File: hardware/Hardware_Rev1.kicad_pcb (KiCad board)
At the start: 2 copper layers, 120.7 x 44.5 mm, 56 parts, among them J1 RJ45_LED_Shielded, J2 6P6C, Q1 BUK9M9R5-40HX, Q2 BUK9M9R5-40HX, Q3 BUK9M9R5-40HX, U1 LT1910, U2 LT1910, U3 OKI, U4 LT1910, U5 TSR_1-2450, U6 Teensy4.1_DEV-16771

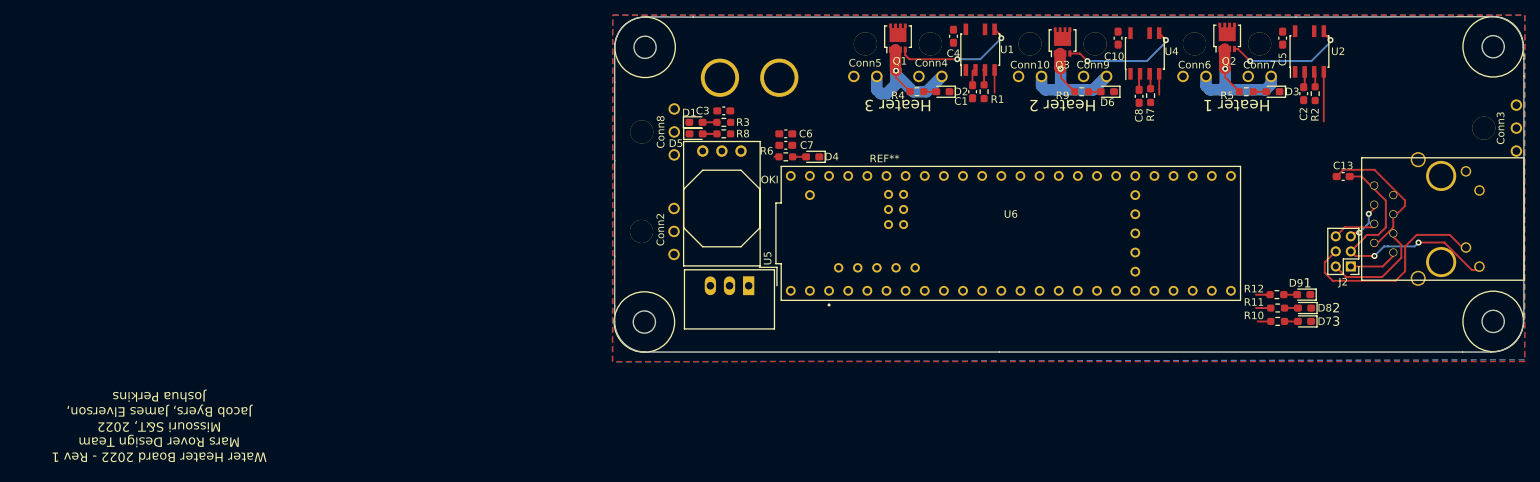
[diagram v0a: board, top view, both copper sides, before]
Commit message: maor
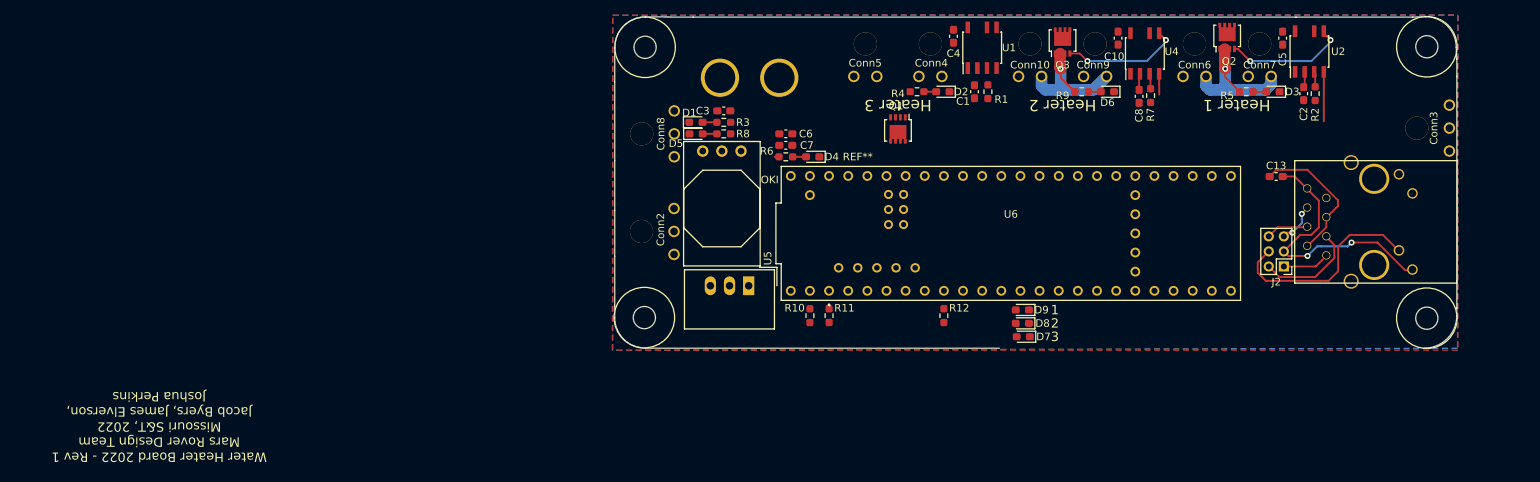
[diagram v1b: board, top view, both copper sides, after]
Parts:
- moved R10 62.1 mm to (114.3, 90.4), turned to 90 degrees
- moved R11 59.5 mm to (116.8, 90.4), turned to 90 degrees
- moved R12 44.3 mm to (132.1, 90.4), turned to 90 degrees
- moved D8 37.5 mm to (142.5, 91.4)
- moved D9 37.4 mm to (142.5, 89.7)
- moved D7 37.4 mm to (142.6, 93.2)
- moved Q1 12.0 mm to (126.0, 65.6), turned to -90 degrees
- moved J1 8.90 mm to (202.2, 77.9)
- moved Conn3 8.89 mm to (200.2, 65.5)
- moved C13 8.89 mm to (176.2, 72.0)
- moved J2 8.89 mm to (177.2, 83.9)
- moved V4 8.82 mm to (192.2, 86.8)
- moved V3 8.81 mm to (192.2, 58.7)
- moved V1 0.59 mm to (96.3, 86.7)
- moved R1 0.51 mm to (137.9, 60.7)
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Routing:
- net Net-(Conn4-Pad1): track 21.6 -> 0.00 mm, vias 1 -> 0
- net Net-(Q1-Pad4): track 16.4 -> 0.00 mm, vias 2 -> 0
- net Heater3: track 3.02 -> 0.00 mm
- net Net-(C1-Pad1): track 2.08 -> 0.00 mm
- net Net-(R1-Pad2): track 2.03 -> 0.00 mm
- net Net-(R11-Pad2): track 1.99 -> 0.00 mm
- net Net-(R12-Pad2): track 1.88 -> 0.00 mm
- net Net-(D8-Pad2): track 1.78 -> 0.00 mm
- net Net-(D9-Pad2): track 1.77 -> 0.00 mm
- net Net-(D7-Pad2): track 1.77 -> 0.00 mm
- net Net-(R10-Pad2): track 1.73 -> 0.00 mm
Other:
- board size 120.7 x 44.5 mm -> 111.8 x 44 mm
